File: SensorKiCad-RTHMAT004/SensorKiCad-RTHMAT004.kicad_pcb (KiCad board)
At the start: 2 copper layers, 102 parts, among them J1 Conn_02x14_Odd_Even, Q1 SS8050, Q2 SS8050, Q3 SS8050, Q4 SS8050, Q5 SS8050, Q6 SS8050

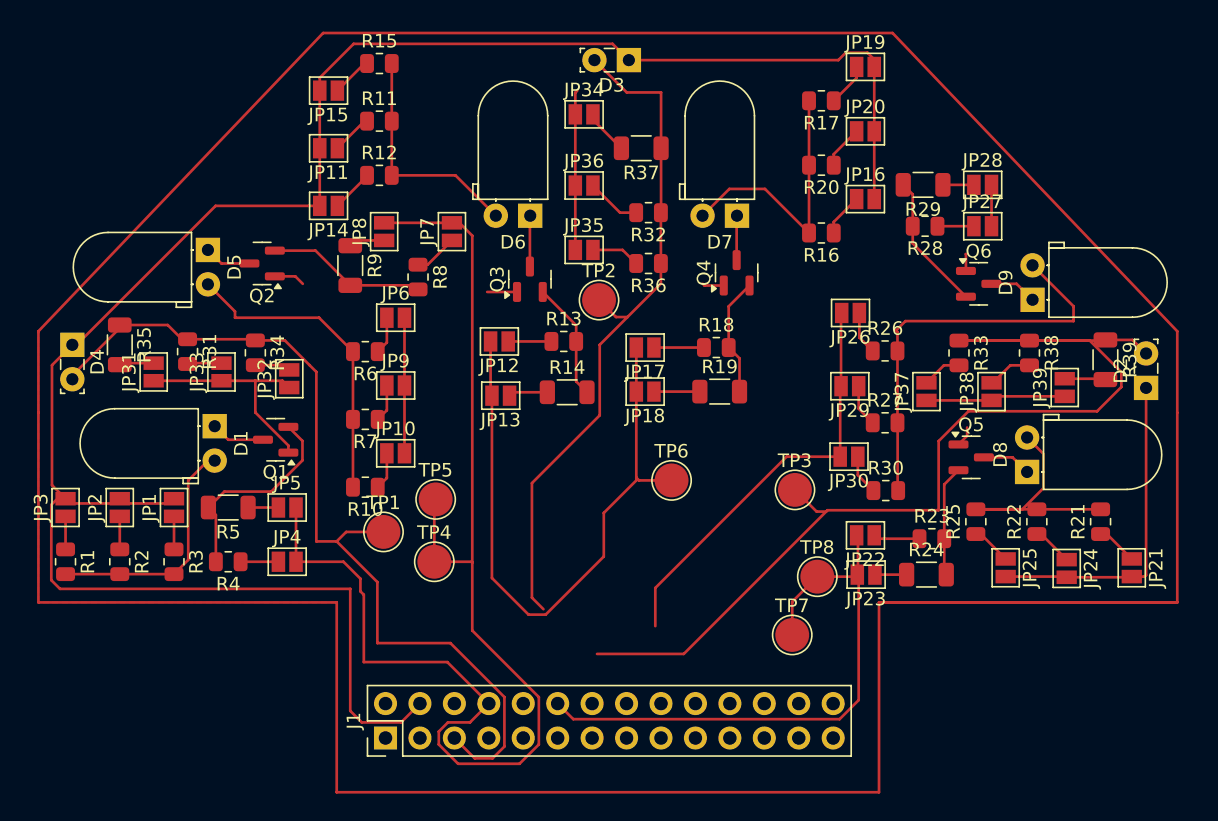
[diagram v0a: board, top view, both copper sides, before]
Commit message: pcb advancements
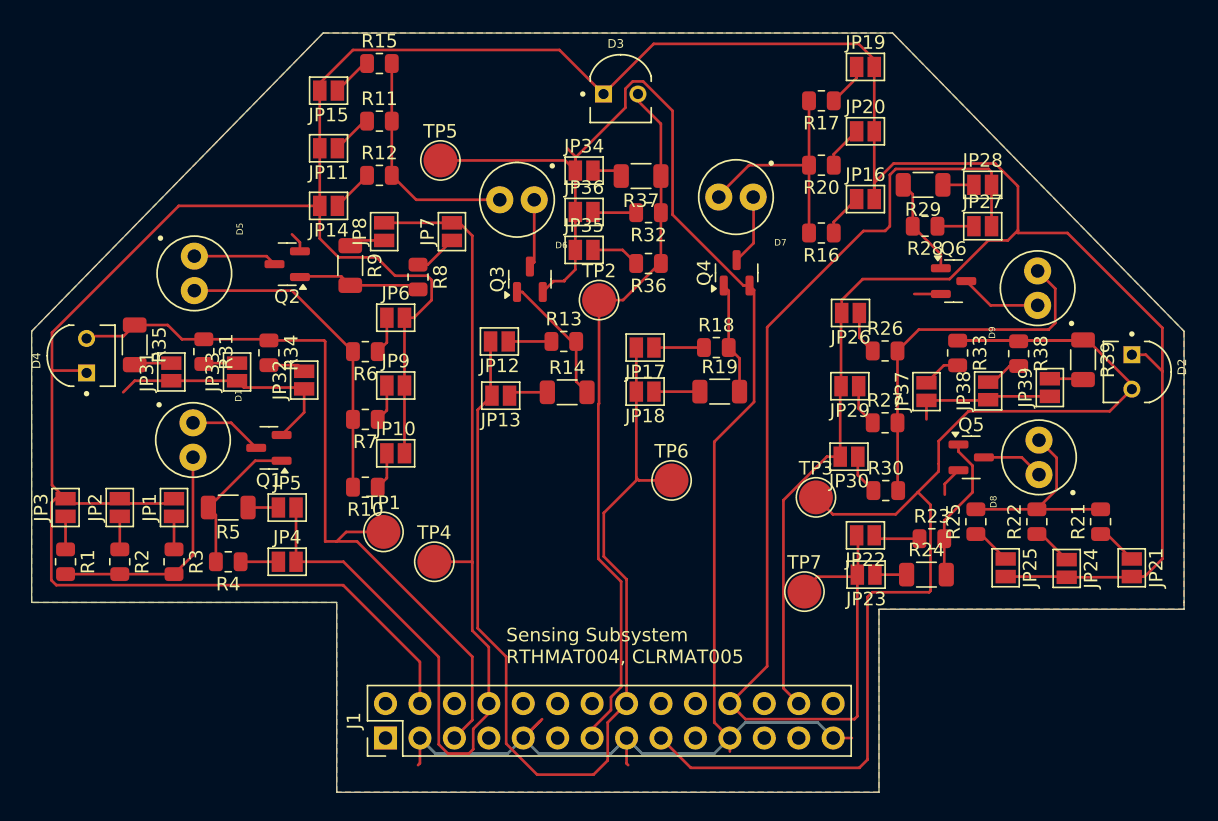
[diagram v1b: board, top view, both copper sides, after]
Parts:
- removed TP8: TestPoint, TestPoint:TestPoint_Pad_D2.5mm
- D1, D5, D6, D7, D8, D9: value SFH4544 -> SFH_4544; footprint LED_THT:LED_D5.0mm_Horizontal_O1.27mm_Z3.0mm_IRBlack -> SFH_4544:DIO_SFH_4544
- D2, D3, D4: footprint LED_THT:LED_SideEmitter_Rectangular_W4.5mm_H1.6mm -> BPV22NF:XDCR_BPV22NF
- moved TP5 25.0 mm to (-32.4, -46.6)
- moved JP34 4.15 mm to (-21.8, -45.9)
- moved TP7 3.32 mm to (-5.50, -14.8)
- moved D3 2.57 mm to (-19.1, -51.5), turned to 0 degrees
- moved R37 2.05 mm to (-17.6, -45.5)
- moved D5 2.00 mm to (-50.5, -38.3)
- moved JP36 1.95 mm to (-21.8, -42.8)
- moved D1 1.90 mm to (-50.6, -26.0)
- moved Q6 1.86 mm to (5.50, -37.7)
- moved Q2 1.85 mm to (-43.6, -39.0)
- moved R39 1.65 mm to (15.1, -31.9)
- moved TP3 1.64 mm to (-4.65, -21.8)
- moved D2 1.58 mm to (18.6, -31.0), turned to -90 degrees
- moved D6 1.53 mm to (-26.7, -43.7)
- moved D8 1.39 mm to (11.8, -24.7)
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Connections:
- J1 pad 10: /PWM Centre -> unconnected-(J1-Pin_10-Pad10)
- J1 pad 11: /Signal Right -> unconnected-(J1-Pin_11-Pad11)
- J1 pad 12: /PWM Right -> unconnected-(J1-Pin_12-Pad12)
- J1 pad 13: unconnected-(J1-Pin_13-Pad13) -> /Signal Centre
- J1 pad 15: unconnected-(J1-Pin_15-Pad15) -> GND
- J1 pad 16: unconnected-(J1-Pin_16-Pad16) -> /PWM Centre
- J1 pad 17: unconnected-(J1-Pin_17-Pad17) -> /Signal Right
- J1 pad 21: unconnected-(J1-Pin_21-Pad21) -> GND
- J1 pad 22: unconnected-(J1-Pin_22-Pad22) -> /PWM Right
- J1 pad 26: unconnected-(J1-Pin_26-Pad26) -> /BATT
- J1 pad 27: unconnected-(J1-Pin_27-Pad27) -> GND
- J1 pad 3: unconnected-(J1-Pin_3-Pad3) -> GND
- J1 pad 7: /Signal Centre -> unconnected-(J1-Pin_7-Pad7)
- Q1 pad 1: GND -> Net-(Q1-B)
- Q1 pad 2: Net-(Q1-B) -> GND
- Q1 pad 3: Net-(D1-K) -> Net-(Q1-C)
- Q2 pad 1: GND -> Net-(Q2-B)
- Q2 pad 2: Net-(Q2-B) -> GND
- Q2 pad 3: Net-(D5-K) -> Net-(Q2-C)
- Q3 pad 1: GND -> Net-(Q3-B)
- Q3 pad 2: Net-(Q3-B) -> GND
- Q3 pad 3: Net-(D6-K) -> Net-(Q3-C)
- Q4 pad 1: GND -> Net-(Q4-B)
- Q4 pad 2: Net-(Q4-B) -> GND
- Q4 pad 3: Net-(D7-K) -> Net-(Q4-C)
- Q5 pad 1: GND -> Net-(Q5-B)
- Q5 pad 2: Net-(Q5-B) -> GND
- Q5 pad 3: Net-(D8-K) -> Net-(Q5-C)
- Q6 pad 1: GND -> Net-(Q6-B)
- Q6 pad 2: Net-(Q6-B) -> GND
- Q6 pad 3: Net-(D9-K) -> Net-(Q6-C)
- R1 pad 2: Net-(D1-A) -> Net-(D1-PadA)
- R10 pad 2: Net-(D5-A) -> Net-(D5-PadA)
- R11 pad 2: Net-(D6-A) -> Net-(D6-PadA)
- R12 pad 2: Net-(D6-A) -> Net-(D6-PadA)
- R15 pad 2: Net-(D6-A) -> Net-(D6-PadA)
- R16 pad 2: Net-(D7-A) -> Net-(D7-PadA)
- R17 pad 2: Net-(D7-A) -> Net-(D7-PadA)
- R2 pad 2: Net-(D1-A) -> Net-(D1-PadA)
- R20 pad 2: Net-(D7-A) -> Net-(D7-PadA)
- R21 pad 2: Net-(D8-A) -> Net-(D8-PadA)
- R22 pad 2: Net-(D8-A) -> Net-(D8-PadA)
- R25 pad 2: Net-(D8-A) -> Net-(D8-PadA)
- R26 pad 2: Net-(D9-A) -> Net-(D9-PadA)
- R27 pad 2: Net-(D9-A) -> Net-(D9-PadA)
- R3 pad 2: Net-(D1-A) -> Net-(D1-PadA)
- R30 pad 2: Net-(D9-A) -> Net-(D9-PadA)
- R6 pad 2: Net-(D5-A) -> Net-(D5-PadA)
- R7 pad 2: Net-(D5-A) -> Net-(D5-PadA)
- TP5 pad 1: /PWM Left -> GND
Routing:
- net GND: track 47.5 -> 164.3 mm
- net /BATT: track 215.8 -> 287.4 mm
- net /PWM Right: track 46.6 -> 84.5 mm
- net Net-(D9-A): track 30.6 -> 0.00 mm
- net /PWM Centre: track 47.7 -> 75.3 mm
- net Net-(D9-PadA): track 0.00 -> 27.2 mm
- net Net-(D5-PadA): track 0.00 -> 23.6 mm
- net Net-(D5-A): track 23.0 -> 0.00 mm
- net Net-(D7-A): track 19.8 -> 0.00 mm
- net Net-(D8-A): track 19.1 -> 0.00 mm
- net /PWM Left: track 94.0 -> 75.4 mm
- net Net-(D1-A): track 17.9 -> 0.00 mm
- net Net-(D7-PadA): track 0.00 -> 17.5 mm
- net Net-(D1-PadA): track 0.00 -> 17.2 mm
- net Net-(D6-A): track 17.2 -> 0.00 mm
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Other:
- board outline added: 85 x 56 mm
- board text added: "Sensing Subsystem RTHMAT004, CLRMAT005"
